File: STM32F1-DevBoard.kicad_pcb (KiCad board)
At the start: 2 copper layers, 20.3 x 50.8 mm, 39 parts, among them J1 USB_C_Receptacle_USB2.0, SW1 SW_Push, SW2 SW_Push, U1 STM32F103C8T6, U2 AMS1117-3.3, U3 W25Q32JVSS

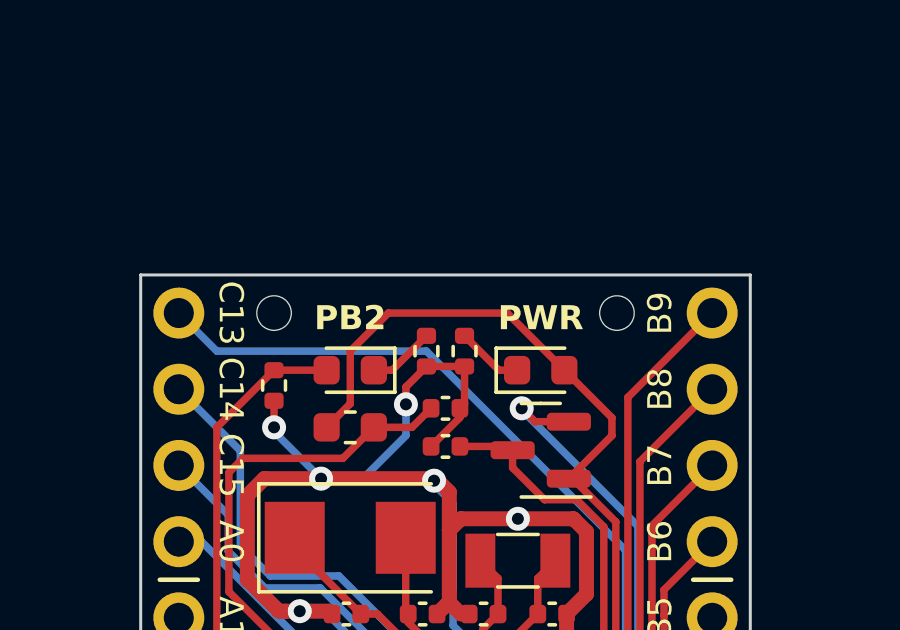
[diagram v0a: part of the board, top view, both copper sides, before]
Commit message: Add files via upload
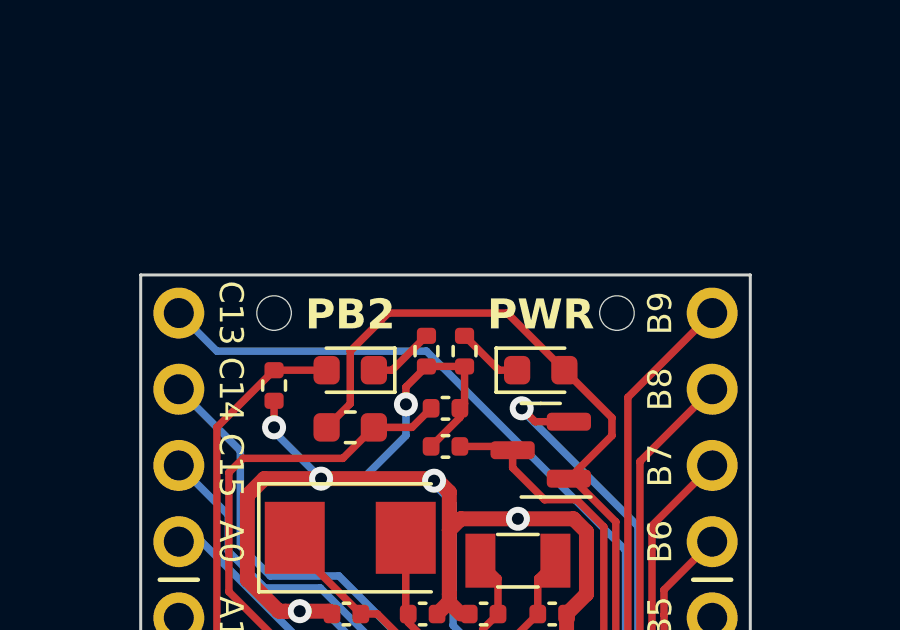
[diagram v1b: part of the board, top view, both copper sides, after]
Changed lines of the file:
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@@
     (descr "SMD Crystal FC-135 https://support.epson.biz/td/api/doc_check.php?dl=brief_FC-135R_en.pdf")
     (tags "SMD SMT Crystal")
-    (property "JLCPCB Rotation Offset" "-180")
+    (property "JLCPCB Rotation Offset" "0")
     (property "LCSC" "C32346")
     (property "Sheetfile" "STM32F1-DevBoard.kicad_sch")
@@
   )
   (gr_text "PB2" (at 133.985 78.105) (layer "F.SilkS")
-    (effects (font (size 0.8 0.8) (thickness 0.15) bold) (justify bottom))
+    (effects (font (size 1 1) (thickness 0.2) bold) (justify bottom))
   )
   (gr_text "A5" (at 129.54 97.79 -90) (layer "F.SilkS")
@@
   )
   (gr_text "PWR" (at 140.335 78.105) (layer "F.SilkS")
-    (effects (font (size 0.8 0.8) (thickness 0.15) bold) (justify bottom))
+    (effects (font (size 1 1) (thickness 0.2) bold) (justify bottom))
   )
   (gr_text "C13" (at 129.54 77.47 -90) (layer "F.SilkS")
